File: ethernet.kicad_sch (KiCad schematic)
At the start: 23 parts, among them J6 RJ45_JK0654219, U20 RTL8153B-VB-CG, Y2 25MHz

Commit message: Add files via upload
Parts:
- C69, C70, C71, C72, C73, C74, C75, C76, C77, C78, C80, C81, C82, C83: footprint (none) -> Capacitor_SMD:C_0603_1608Metric
- C79: footprint (none) -> Capacitor_SMD:C_1206_3216Metric
- L3, R24, R25, R26, R27: footprint (none) -> Resistor_SMD:R_0603_1608Metric
- Y2: footprint (none) -> Crystal:Crystal_SMD_3225-4Pin_3.2x2.5mm
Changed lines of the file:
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@@
 			)
 		)
-		(property "Footprint" ""
+		(property "Footprint" "Capacitor_SMD:C_0603_1608Metric"
 			(at 243.84 74.93 0)
 			(hide yes)
@@
 			)
 		)
-		(property "Footprint" ""
+		(property "Footprint" "Resistor_SMD:R_0603_1608Metric"
 			(at 128.27 96.52 0)
 			(hide yes)
@@
 			)
 		)
-		(property "Footprint" ""
+		(property "Footprint" "Capacitor_SMD:C_0603_1608Metric"
 			(at 121.92 76.2 0)
 			(hide yes)
@@
 			)
 		)
-		(property "Footprint" ""
+		(property "Footprint" "Capacitor_SMD:C_0603_1608Metric"
 			(at 76.2 138.43 0)
 			(hide yes)
@@
 			)
 		)
-		(property "Footprint" ""
+		(property "Footprint" "Capacitor_SMD:C_0603_1608Metric"
 			(at 132.08 76.2 0)
 			(hide yes)
@@
 			)
 		)
-		(property "Footprint" ""
+		(property "Footprint" "Resistor_SMD:R_0603_1608Metric"
 			(at 209.55 104.14 0)
 			(hide yes)
@@
 			)
 		)
-		(property "Footprint" ""
+		(property "Footprint" "Crystal:Crystal_SMD_3225-4Pin_3.2x2.5mm"
 			(at 127 71.12 0)
 			(hide yes)
@@
 			)
 		)
-		(property "Footprint" ""
+		(property "Footprint" "Capacitor_SMD:C_0603_1608Metric"
 			(at 227.33 129.54 0)
 			(hide yes)
@@
 			)
 		)
-		(property "Footprint" ""
+		(property "Footprint" "Capacitor_SMD:C_0603_1608Metric"
 			(at 222.25 76.2 0)
 			(hide yes)
@@
 			)
 		)
-		(property "Footprint" ""
+		(property "Footprint" "Capacitor_SMD:C_0603_1608Metric"
 			(at 228.6 68.58 0)
 			(hide yes)
@@
 			)
 		)
-		(property "Footprint" ""
+		(property "Footprint" "Capacitor_SMD:C_0603_1608Metric"
 			(at 228.6 81.28 0)
 			(hide yes)
@@
 			)
 		)
-		(property "Footprint" ""
+		(property "Footprint" "Capacitor_SMD:C_0603_1608Metric"
 			(at 231.14 100.33 0)
 			(hide yes)
@@
 			)
 		)
-		(property "Footprint" ""
+		(property "Footprint" "Capacitor_SMD:C_0603_1608Metric"
 			(at 243.84 82.55 0)
 			(hide yes)
@@
 			)
 		)
-		(property "Footprint" ""
+		(property "Footprint" "Capacitor_SMD:C_0603_1608Metric"
 			(at 222.25 83.82 0)
 			(hide yes)
@@
 			)
 		)
-		(property "Footprint" ""
+		(property "Footprint" "Capacitor_SMD:C_0603_1608Metric"
 			(at 228.6 73.66 0)
 			(hide yes)
@@
 			)
 		)
-		(property "Footprint" ""
+		(property "Footprint" "Resistor_SMD:R_0603_1608Metric"
 			(at 209.55 101.6 0)
 			(hide yes)
@@
 			)
 		)
-		(property "Footprint" ""
+		(property "Footprint" "Capacitor_SMD:C_0603_1608Metric"
 			(at 220.98 132.08 0)
 			(hide yes)
@@
 			)
 		)
-		(property "Footprint" ""
+		(property "Footprint" "Capacitor_SMD:C_0603_1608Metric"
 			(at 106.68 120.65 0)
 			(hide yes)
@@
 			)
 		)
-		(property "Footprint" ""
+		(property "Footprint" "Resistor_SMD:R_0603_1608Metric"
 			(at 218.44 96.52 0)
 			(hide yes)
@@
 			)
 		)
-		(property "Footprint" ""
+		(property "Footprint" "Capacitor_SMD:C_1206_3216Metric"
 			(at 223.52 100.33 0)
 			(hide yes)
@@
 			)
 		)
-		(property "Footprint" ""
+		(property "Footprint" "Resistor_SMD:R_0603_1608Metric"
 			(at 71.12 138.43 0)
 			(hide yes)

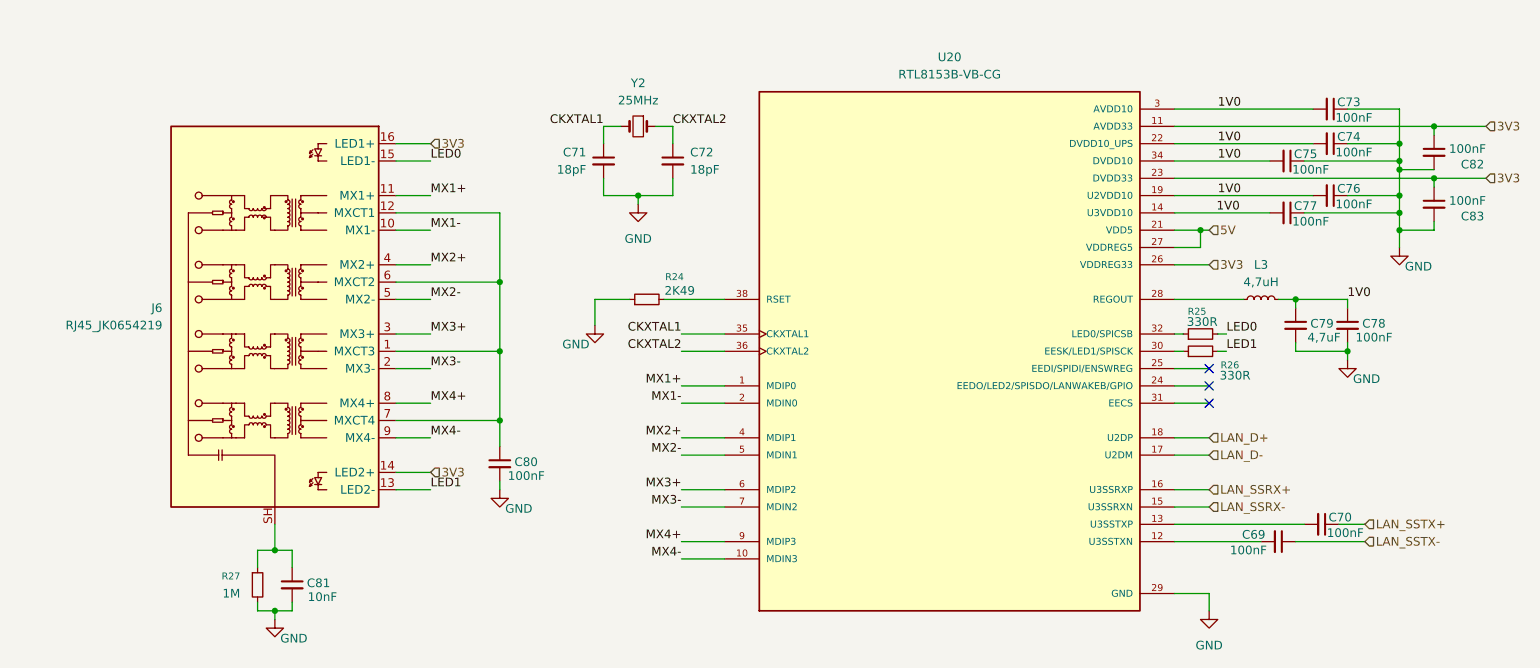
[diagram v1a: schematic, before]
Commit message: Add files via upload
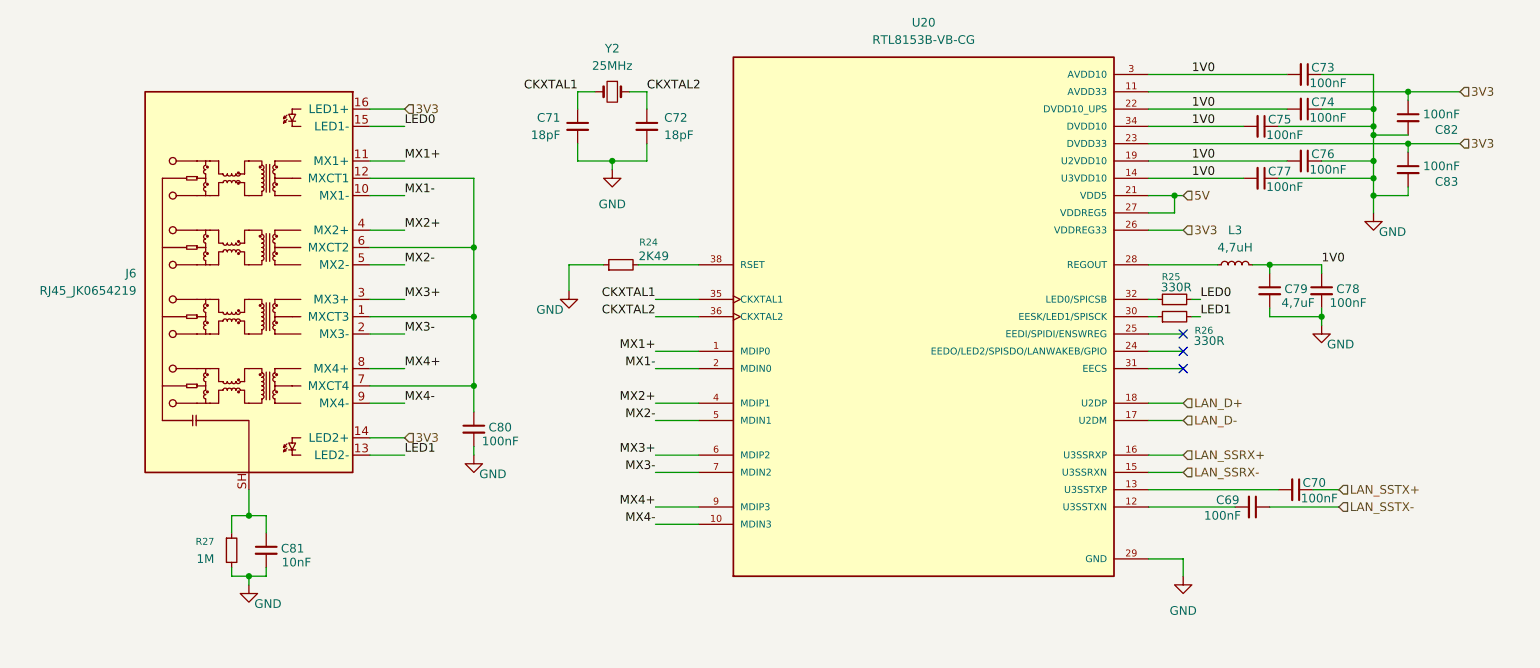
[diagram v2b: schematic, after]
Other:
- moved on the sheet: C69, C70, C71, C72, C73, C74, C75, C76, C77, C78, C79, C80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
